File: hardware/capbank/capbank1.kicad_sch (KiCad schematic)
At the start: 12 parts, among them J1 Screws, U5 PAI130M61

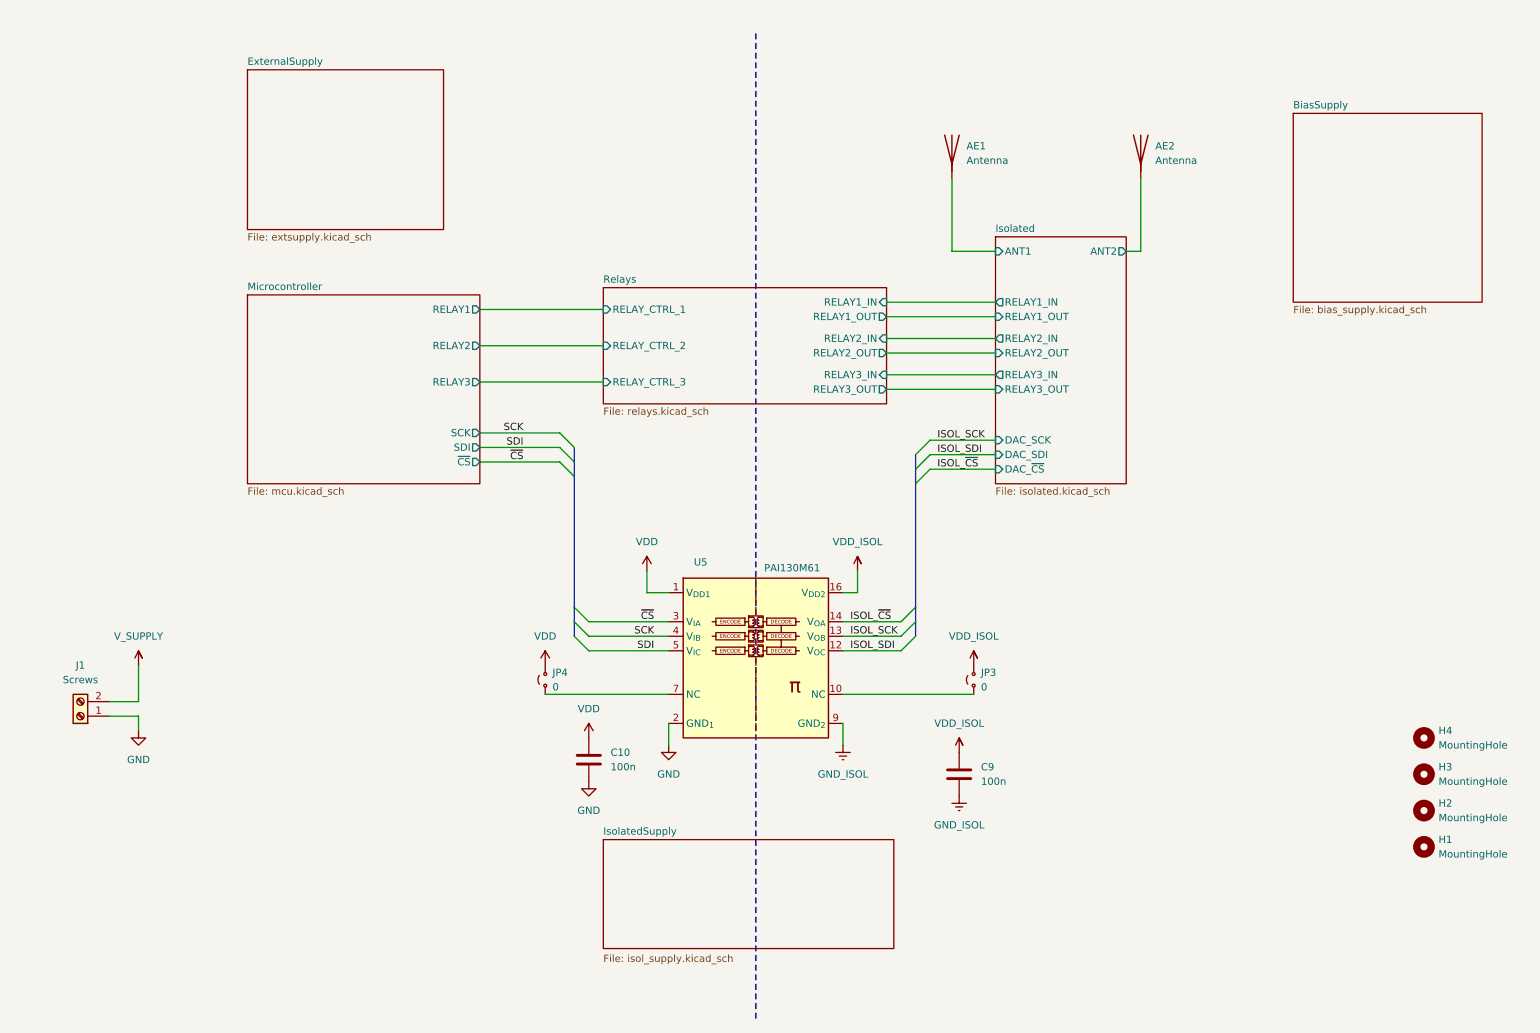
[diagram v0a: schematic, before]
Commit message: Small hardware changes
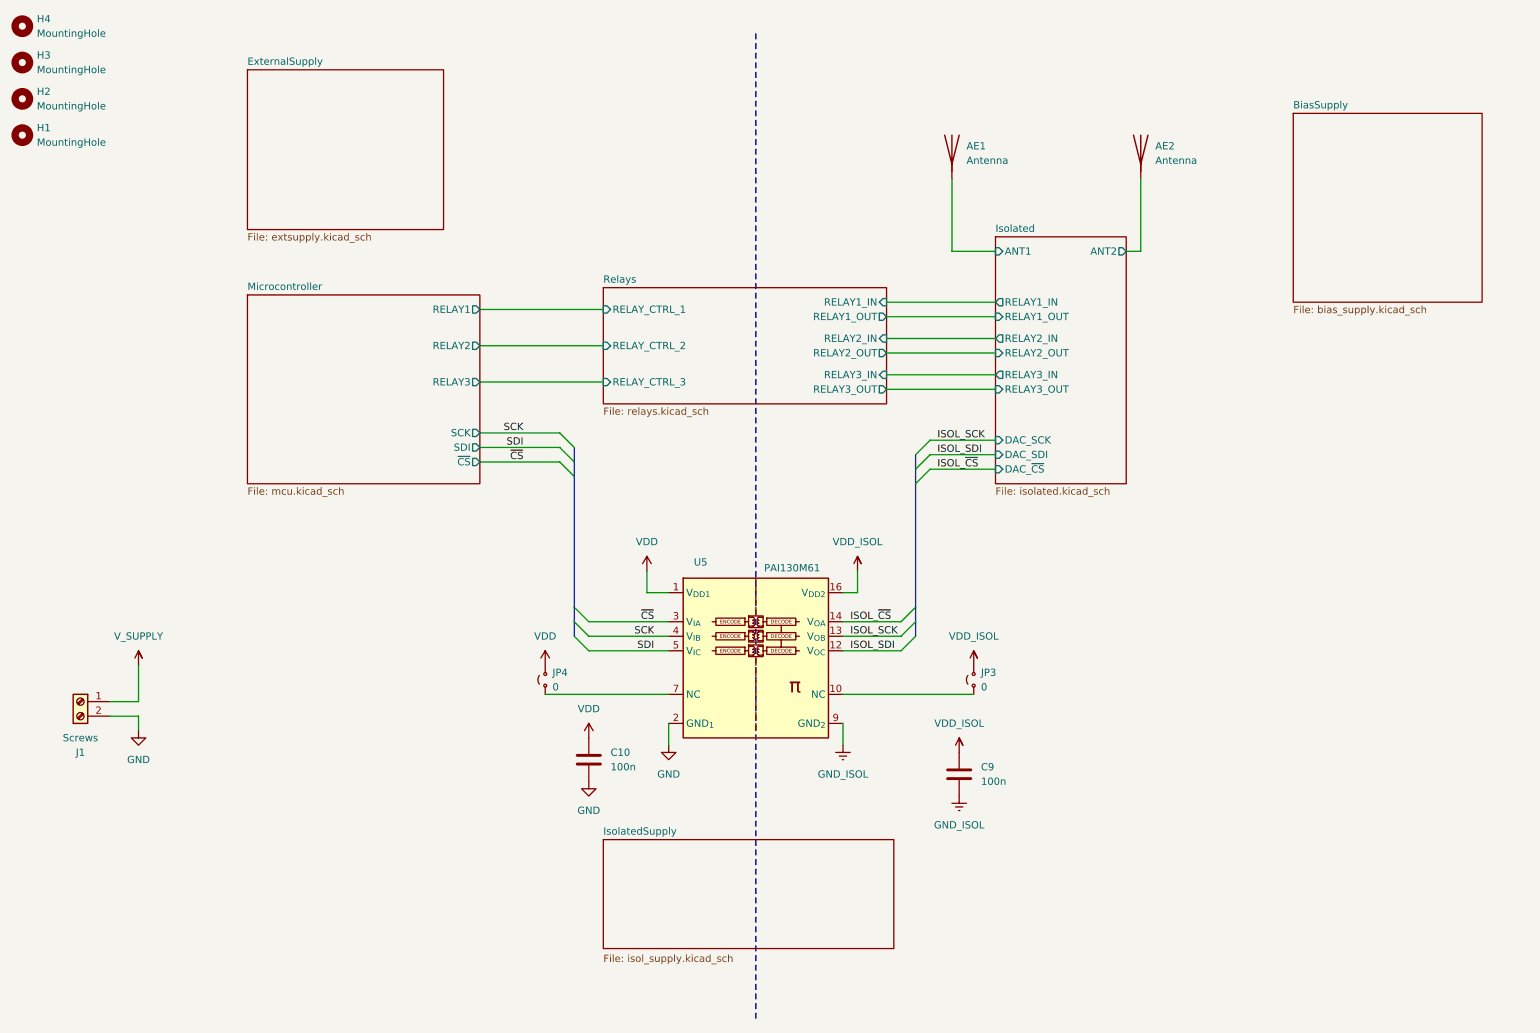
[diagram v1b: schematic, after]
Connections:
- net GND: now also J1.2 (Pin_2); no longer J1.1 (Pin_1)
- net V_SUPPLY: now also J1.1 (Pin_1); no longer J1.2 (Pin_2)
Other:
- moved on the sheet: H1, H2, H3, H4, J1
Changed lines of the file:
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@@
 	(symbol
 		(lib_id "Mechanical:MountingHole")
-		(at 262.89 140.97 0)
+		(at 17.78 16.51 0)
 		(unit 1)
 		(exclude_from_sim no)
@@
 		(on_board yes)
 		(dnp no)
-		(fields_autoplaced yes)
 		(property "Reference" "H4"
-			(at 265.43 139.6999 0)
+			(at 20.32 15.2399 0)
 			(effects
 				(font
@@
 		)
 		(property "Value" "MountingHole"
-			(at 265.43 142.2399 0)
+			(at 20.32 17.7799 0)
 			(effects
 				(font
@@
 		)
 		(property "Footprint" "MountingHole:MountingHole_3.2mm_M3"
-			(at 262.89 140.97 0)
+			(at 17.78 16.51 0)
 			(effects
 				(font
@@
 		)
 		(property "Datasheet" "~"
-			(at 262.89 140.97 0)
+			(at 17.78 16.51 0)
 			(effects
 				(font
@@
 		)
 		(property "Description" "Mounting Hole without connection"
-			(at 262.89 140.97 0)
+			(at 17.78 16.51 0)
 			(effects
 				(font
@@
 	(symbol
 		(lib_id "Mechanical:MountingHole")
-		(at 262.89 160.02 0)
+		(at 17.78 35.56 0)
 		(unit 1)
 		(exclude_from_sim no)
@@
 		(on_board yes)
 		(dnp no)
-		(fields_autoplaced yes)
 		(property "Reference" "H1"
-			(at 265.43 158.7499 0)
+			(at 20.32 34.2899 0)
 			(effects
 				(font
@@
 		)
 		(property "Value" "MountingHole"
-			(at 265.43 161.2899 0)
+			(at 20.32 36.8299 0)
 			(effects
 				(font
@@
 		)
 		(property "Footprint" "MountingHole:MountingHole_3.2mm_M3"
-			(at 262.89 160.02 0)
+			(at 17.78 35.56 0)
 			(effects
 				(font
@@
 		)
 		(property "Datasheet" "~"
-			(at 262.89 160.02 0)
+			(at 17.78 35.56 0)
 			(effects
 				(font
@@
 		)
 		(property "Description" "Mounting Hole without connection"
-			(at 262.89 160.02 0)
+			(at 17.78 35.56 0)
 			(effects
 				(font
@@
 	(symbol
 		(lib_id "Mechanical:MountingHole")
-		(at 262.89 147.32 0)
+		(at 17.78 22.86 0)
 		(unit 1)
 		(exclude_from_sim no)
@@
 		(on_board yes)
 		(dnp no)
-		(fields_autoplaced yes)
 		(property "Reference" "H3"
-			(at 265.43 146.0499 0)
+			(at 20.32 21.5899 0)
 			(effects
 				(font
@@
 		)
 		(property "Value" "MountingHole"
-			(at 265.43 148.5899 0)
+			(at 20.32 24.1299 0)
 			(effects
 				(font
@@
 		)
 		(property "Footprint" "MountingHole:MountingHole_3.2mm_M3"
-			(at 262.89 147.32 0)
+			(at 17.78 22.86 0)
 			(effects
 				(font
@@
 		)
 		(property "Datasheet" "~"
-			(at 262.89 147.32 0)
+			(at 17.78 22.86 0)
 			(effects
 				(font
@@
 		)
 		(property "Description" "Mounting Hole without connection"
-			(at 262.89 147.32 0)
+			(at 17.78 22.86 0)
 			(effects
 				(font
@@
 	(symbol
 		(lib_id "Connector:Screw_Terminal_01x02")
-		(at 27.94 137.16 180)
+		(at 27.94 134.62 0)
+		(mirror y)
 		(unit 1)
 		(exclude_from_sim no)
@@
 		(on_board yes)
 		(dnp no)
-		(fields_autoplaced yes)
 		(property "Reference" "J1"
-			(at 27.94 128.27 0)
+			(at 27.94 143.51 0)
 			(effects
 				(font
@@
 		)
 		(property "Value" "Screws"
-			(at 27.94 130.81 0)
+			(at 27.94 140.97 0)
 			(effects
 				(font
@@
 		)
 		(property "Footprint" "TerminalBlock_Phoenix:TerminalBlock_Phoenix_MPT-0,5-2-2.54_1x02_P2.54mm_Horizontal"
-			(at 27.94 137.16 0)
+			(at 27.94 134.62 0)
 			(effects
 				(font
@@
 		)
 		(property "Datasheet" "~"
-			(at 27.94 137.16 0)
+			(at 27.94 134.62 0)
 			(effects
 				(font
@@
 		)
 		(property "Description" "Generic screw terminal, single row, 01x02, script generated (kicad-library-utils/schlib/autogen/connector/)"
-			(at 27.94 137.16 0)
+			(at 27.94 134.62 0)
 			(effects
 				(font
@@
 	(symbol
 		(lib_id "Mechanical:MountingHole")
-		(at 262.89 153.67 0)
+		(at 17.78 29.21 0)
 		(unit 1)
 		(exclude_from_sim no)
@@
 		(on_board yes)
 		(dnp no)
-		(fields_autoplaced yes)
 		(property "Reference" "H2"
-			(at 265.43 152.3999 0)
+			(at 20.32 27.9399 0)
 			(effects
 				(font
@@
 		)
 		(property "Value" "MountingHole"
-			(at 265.43 154.9399 0)
+			(at 20.32 30.4799 0)
 			(effects
 				(font
@@
 		)
 		(property "Footprint" "MountingHole:MountingHole_3.2mm_M3"
-			(at 262.89 153.67 0)
+			(at 17.78 29.21 0)
 			(effects
 				(font
@@
 		)
 		(property "Datasheet" "~"
-			(at 262.89 153.67 0)
+			(at 17.78 29.21 0)
 			(effects
 				(font
@@
 		)
 		(property "Description" "Mounting Hole without connection"
-			(at 262.89 153.67 0)
-			(effects
-				(font
+			(at 17.78 29.21 0)
+			(effects
+				(font

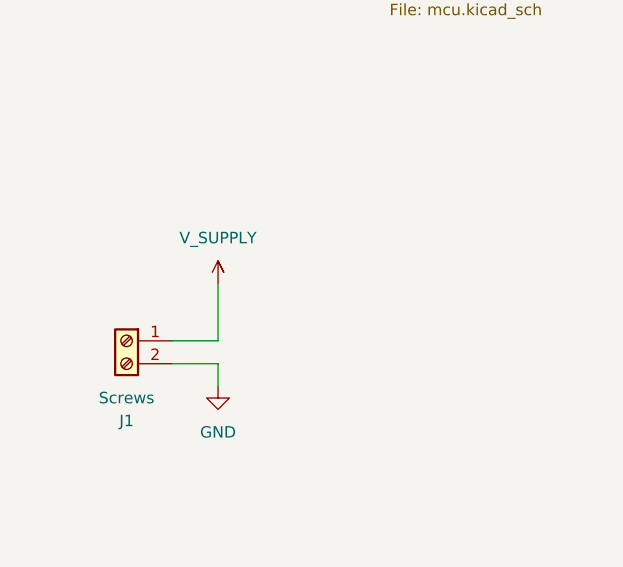
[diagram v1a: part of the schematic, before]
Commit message: Update PCB with learned lessons
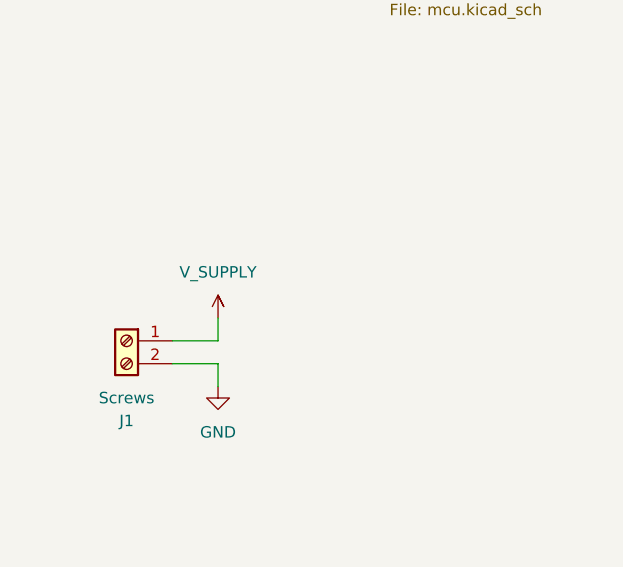
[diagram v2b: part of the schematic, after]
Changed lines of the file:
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@@
 	(wire
 		(pts
-			(xy 38.1 128.27) (xy 38.1 134.62)
+			(xy 38.1 132.08) (xy 38.1 134.62)
 		)
 		(stroke
@@
 	(symbol
 		(lib_id "proj_power:V_SUPPLY")
-		(at 38.1 128.27 0)
+		(at 38.1 132.08 0)
 		(unit 1)
 		(exclude_from_sim no)
@@
 		(fields_autoplaced yes)
 		(property "Reference" "#PWR034"
-			(at 38.1 128.27 0)
+			(at 38.1 132.08 0)
 			(effects
 				(font
@@
 		)
 		(property "Value" "V_SUPPLY"
-			(at 38.1 123.19 0)
+			(at 38.1 127 0)
 			(effects
 				(font
@@
 		)
 		(property "Footprint" ""
-			(at 38.1 128.27 0)
+			(at 38.1 132.08 0)
 			(effects
 				(font
@@
 		)
 		(property "Datasheet" ""
-			(at 38.1 128.27 0)
+			(at 38.1 132.08 0)
 			(effects
 				(font
@@
 		)
 		(property "Description" ""
-			(at 38.1 128.27 0)
-			(effects
-				(font
+			(at 38.1 132.08 0)
+			(effects
+				(font
